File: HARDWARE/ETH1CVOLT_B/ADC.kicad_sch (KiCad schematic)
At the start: 20 parts, among them U4 DG412LEDQ, U5 LTC2400, U6 LT1077S8#TRPBF, U7 AD8475xRMZ, U8 ADA4522-1ARMZ

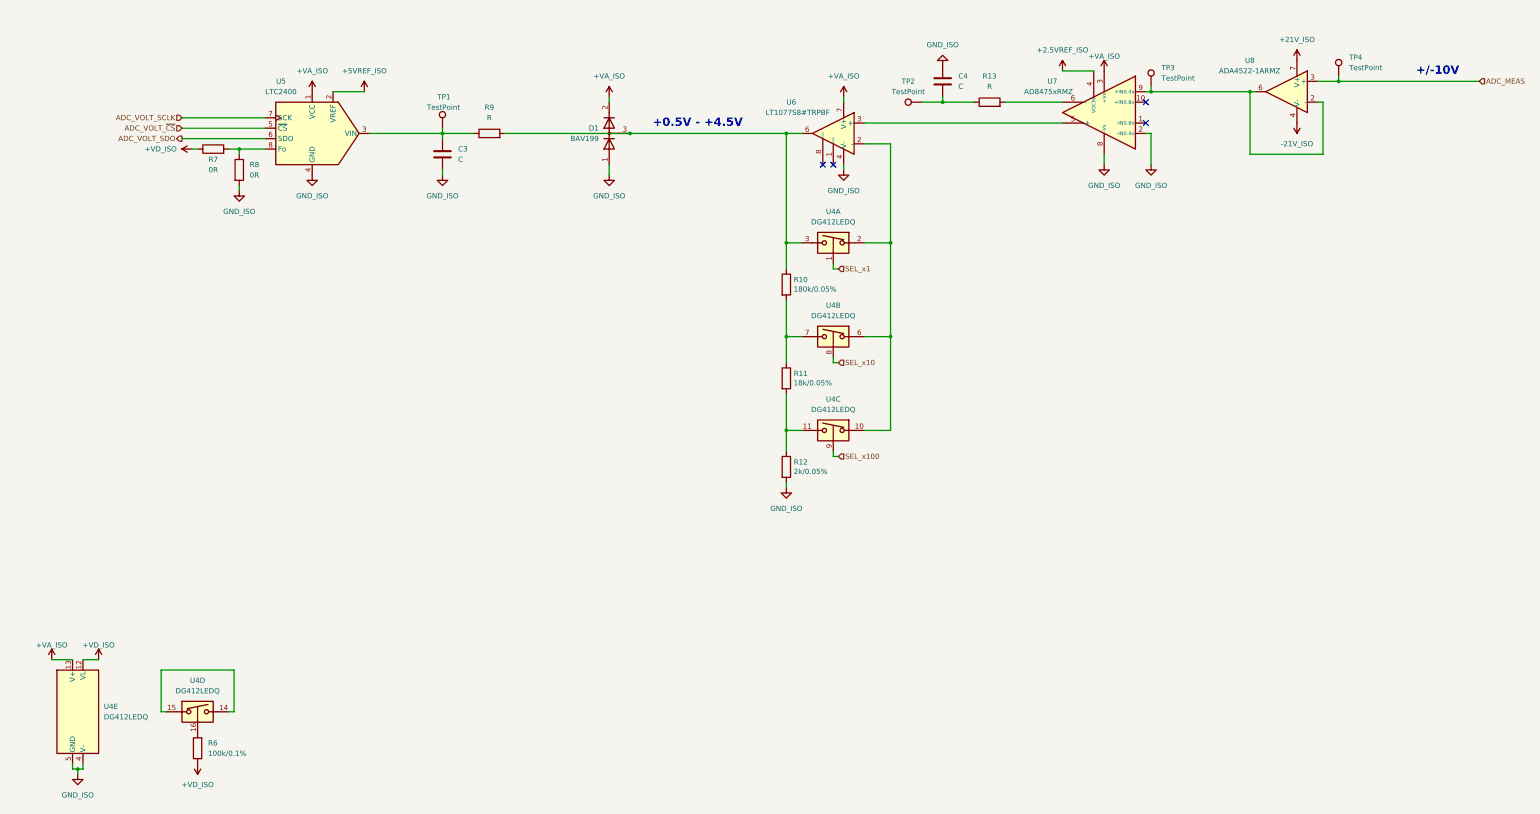
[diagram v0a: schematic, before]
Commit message: Development
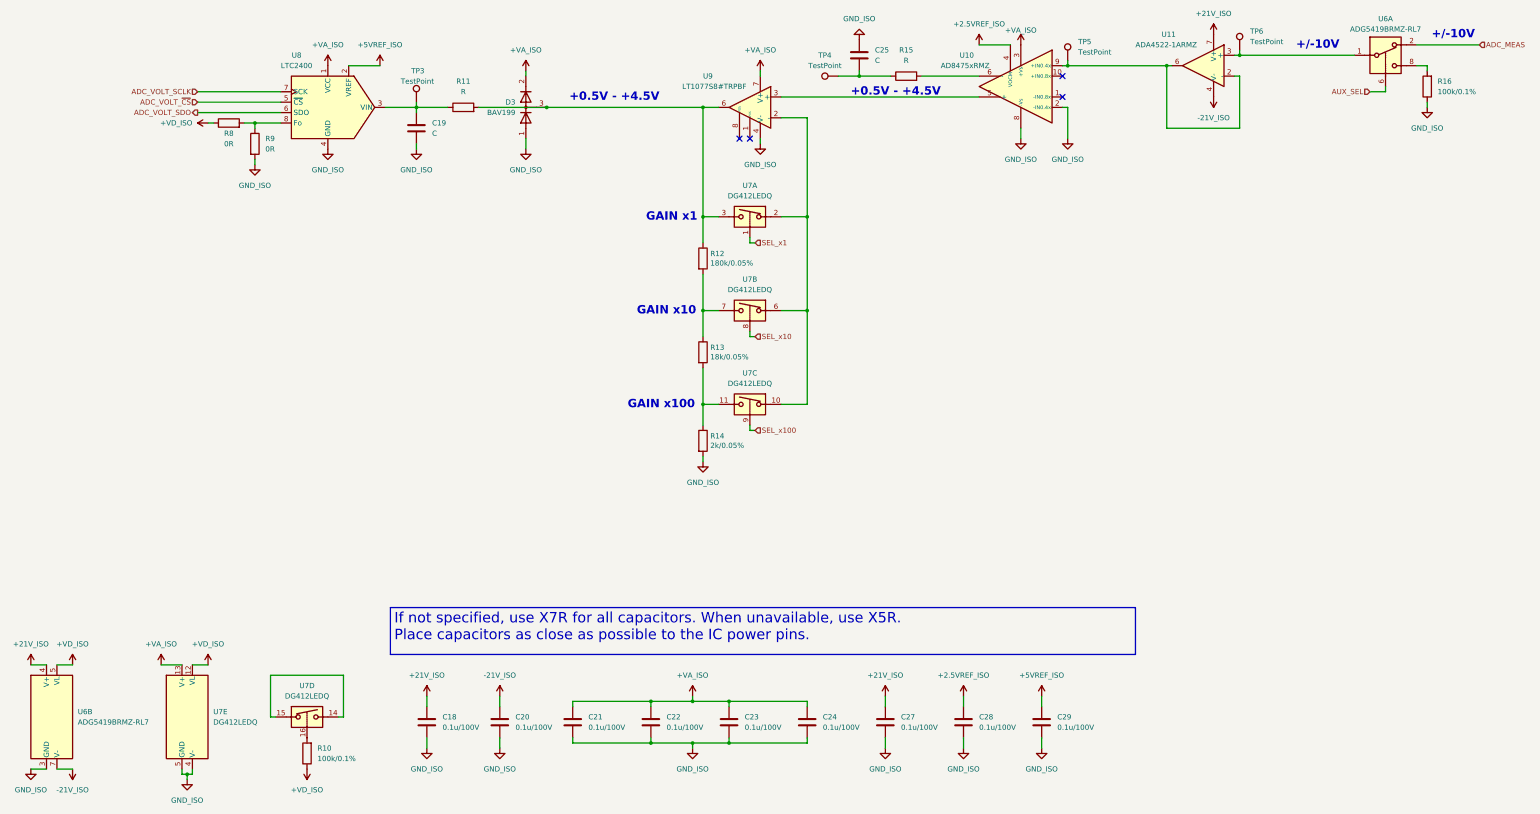
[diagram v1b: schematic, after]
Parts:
- added C18, C20, C21, C22, C23, C24, C27, C28, C29: 0.1u/100V, symbol Device:C
- added R16: 100k/0.1%, Resistor_SMD:R_0603_1608Metric_Pad0.98x0.95mm_HandSolder, symbol Device:R
- added U6: ADG5419BRMZ-RL7, Package_SO:MSOP-8_3x3mm_P0.65mm, symbol Analog_Switch:ADG419BR
- renumbered C3 to C19, C4 to C25, D1 to D3, R6 to R10, R9 to R11, R10 to R12, R11 to R13, R12 to R14, R13 to R15, R7 to R8, R8 to R9, TP1 to TP3, TP2 to TP4, TP3 to TP5, TP4 to TP6, U7 to U10, U8 to U11, U4 to U7, U5 to U8, U6 to U9
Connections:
- net +2.5VREF_ISO: now also C28.1
- net +21V_ISO: now also C18.1, C27.1, U6.4 (V+)
- net +5VREF_ISO: now also C29.1
- net +VA_ISO: now also C21.1, C22.1, C23.1, C24.1
- net +VD_ISO: now also U6.5 (VL)
- net -21V_ISO: now also C20.1, U6.7 (V-)
- net ADC_MEAS: now also U6.2; no longer TP6.1, U11.3 (+)
- net GND_ISO: now also C18.2, C20.2, C21.2, C22.2, C23.2, C24.2, C27.2, C28.2, C29.2, R16.1, U6.3 (GND)
- new net: TP6.1, U11.3 (+), U6.1
- new net: R16.2, U6.8
- new net AUX_SEL: U6.6
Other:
- note added: "GAIN x1"
- note added: "GAIN x10"
- note added: "GAIN x100"
- moved on the sheet: C19, C25, D3, R10, R11, R12, R13, R14, R15, R8, R9, TP3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
